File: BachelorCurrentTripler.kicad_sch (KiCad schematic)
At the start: 7 parts, among them J1 Conn_01x07_Pin, J2 Conn_01x01_Pin, J3 Conn_01x01_Pin, J4 Conn_01x04_Socket, J5 Conn_01x01_Pin

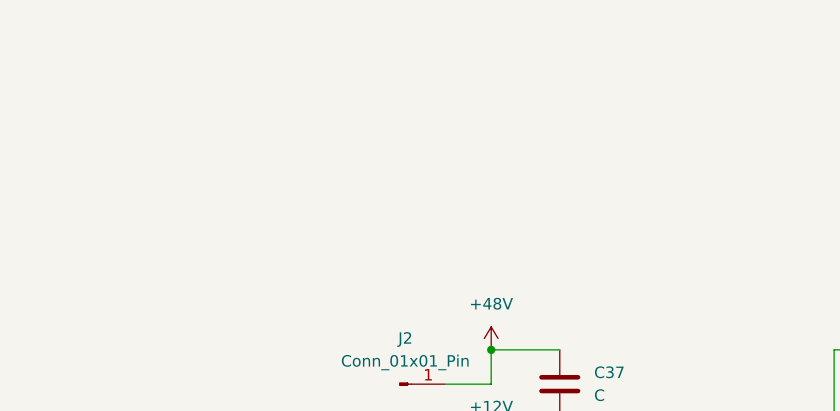
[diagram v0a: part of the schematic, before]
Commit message: Rettelser efter møde med Andreas
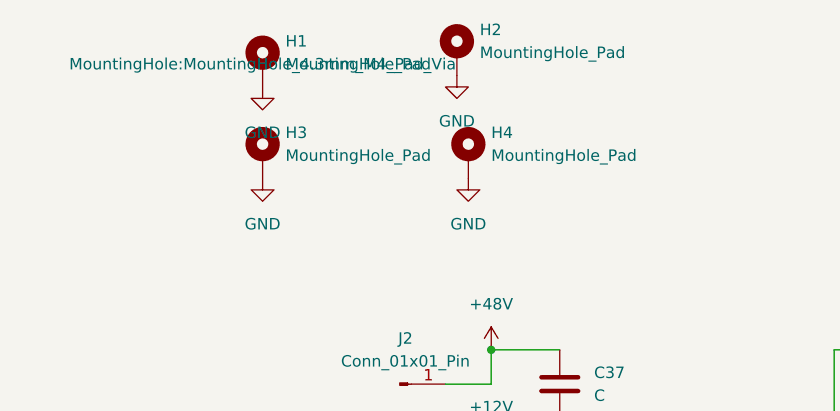
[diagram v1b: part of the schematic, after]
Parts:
- added H1, H2, H3, H4: MountingHole_Pad, MountingHole:MountingHole_4.3mm_M4_Pad_Via, symbol Mechanical:MountingHole_Pad
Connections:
- net GND: now also H1.1, H2.1, H3.1, H4.1
